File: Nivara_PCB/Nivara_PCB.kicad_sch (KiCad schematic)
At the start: 19 parts, among them J1 NPN_IN, J10 RELAY, J11 FUENTE IN, J12 FUENTE EX, J2 PNP_IN, J3 D_IN, J4 ANALOG_IN, J5 RUN/STOP, J6 NPN_OUT, J7 PNP_OUT, J8 RS485, J9 ANALOG_OUT

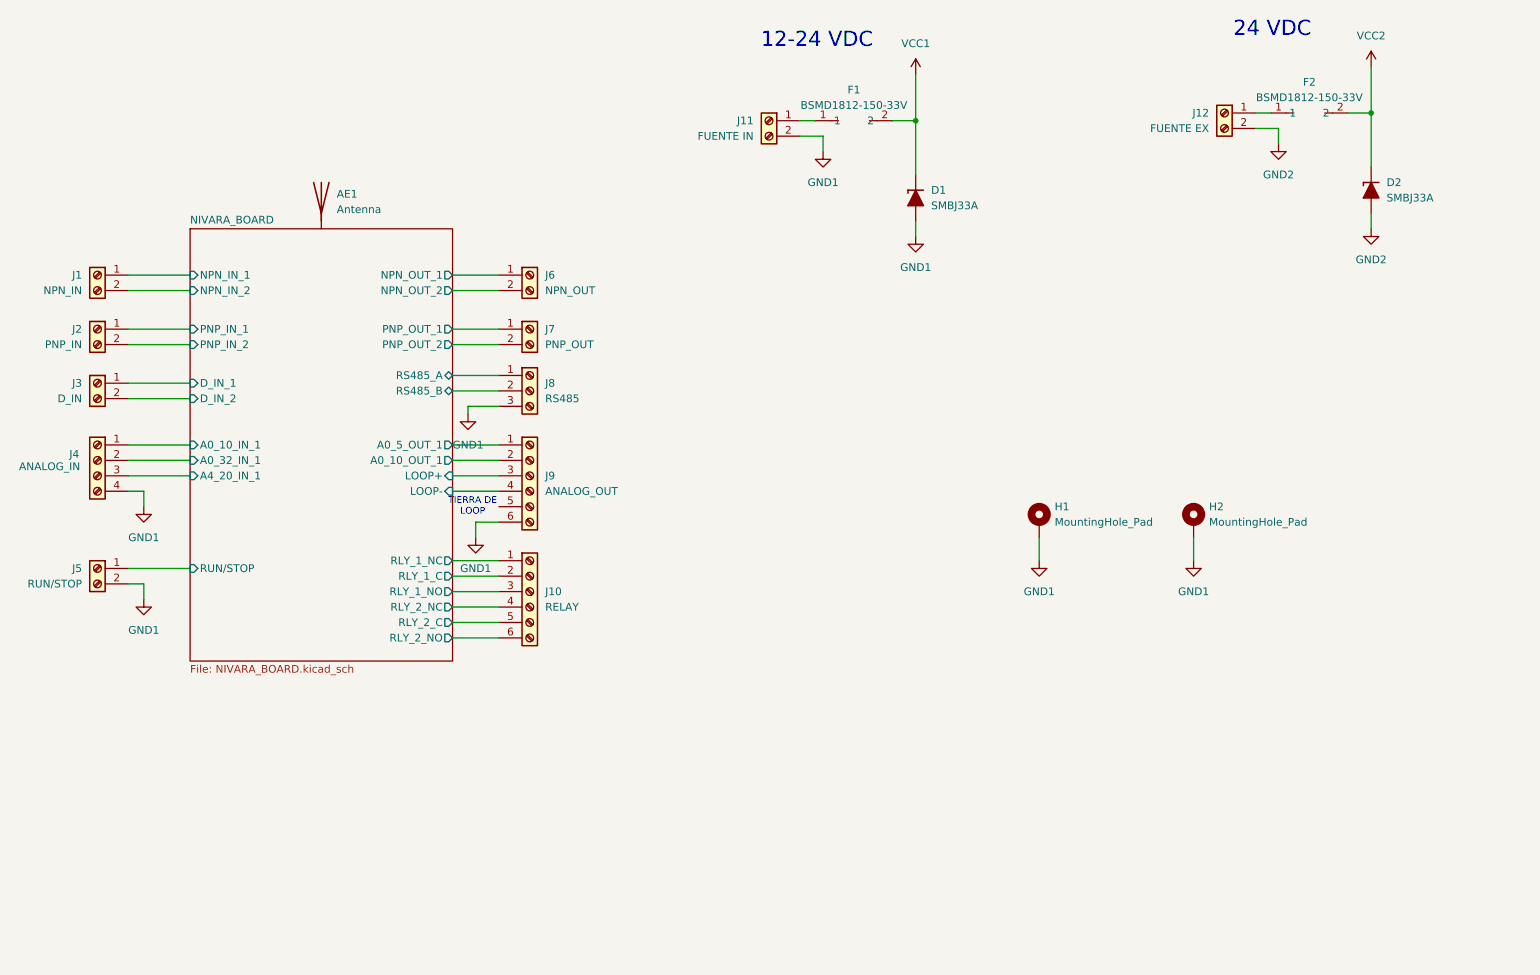
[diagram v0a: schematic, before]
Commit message: New changes to the Nivara PCB schematic files.
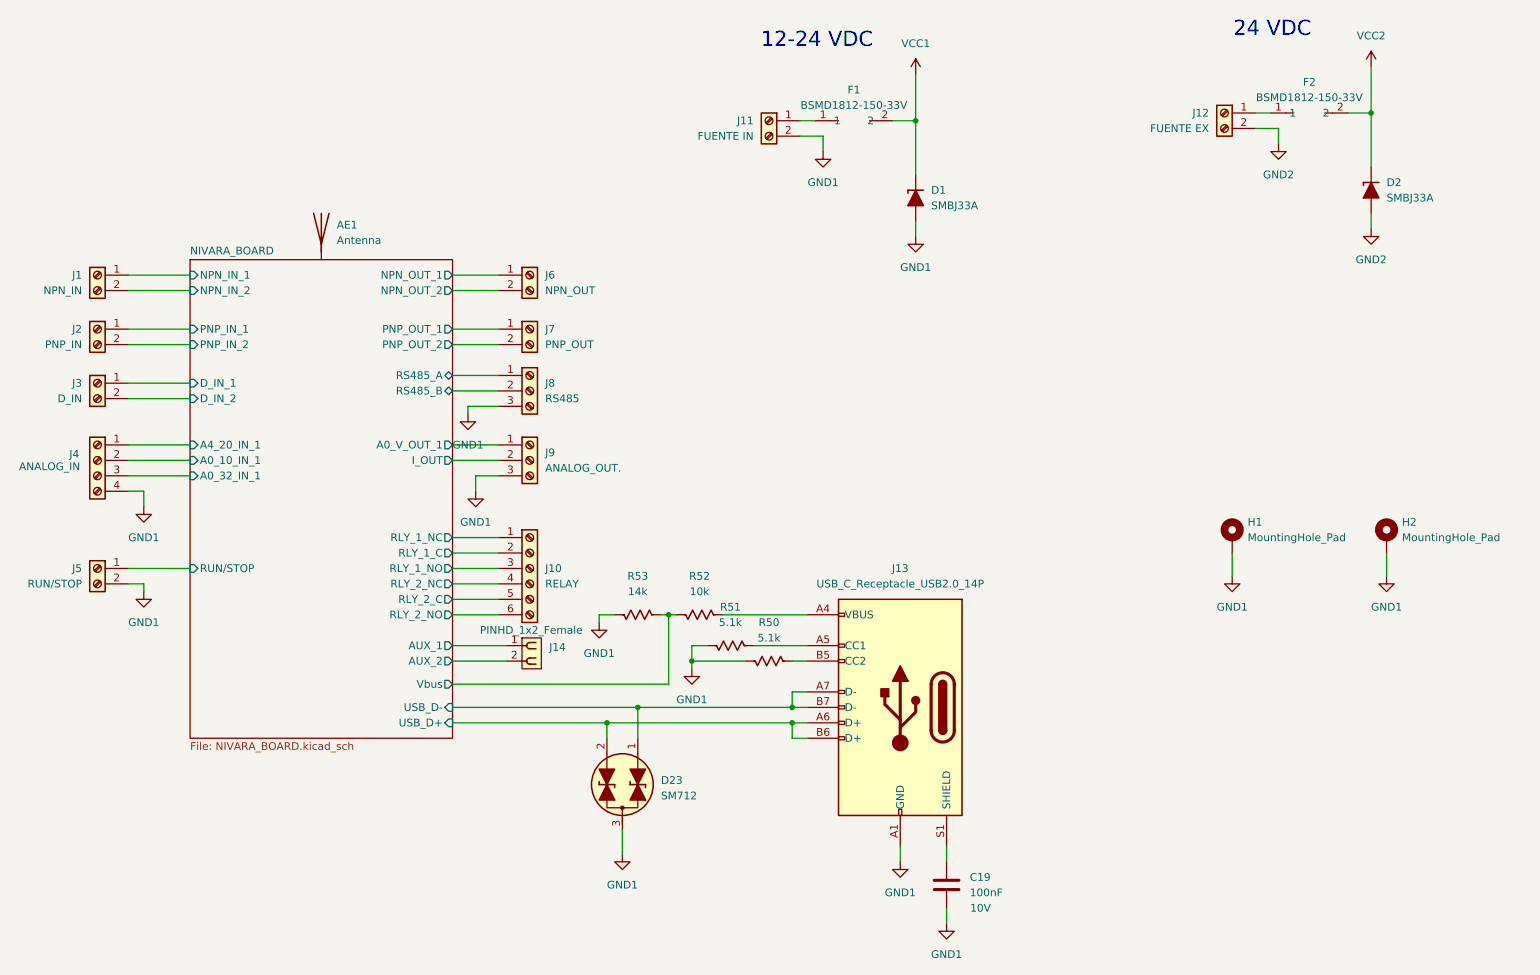
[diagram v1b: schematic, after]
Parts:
- removed J9: ANALOG_OUT, TerminalBlock:TerminalBlock_bornier-6_P5.08mm, symbol Connector:Screw_Terminal_01x06
- added C19: 100nF, PCM_Capacitor_SMD_AKL:C_0603_1608Metric, symbol PCM_Capacitor_US_AKL:C_0603
- added D23: SM712, PCM_Package_TO_SOT_SMD_AKL:SOT-23, symbol PCM_Diode_TVS_AKL:SM712
- added J13: USB_C_Receptacle_USB2.0_14P, symbol Connector:USB_C_Receptacle_USB2.0_14P
- added J14: PINHD_1x2_Female, Connector_PinSocket_2.54mm:PinSocket_1x02_P2.54mm_Vertical, symbol PCM_SL_Pin_Headers:PINHD_1x2_Female
- added J9: ANALOG_OUT., TerminalBlock:TerminalBlock_bornier-3_P5.08mm, symbol Connector:Screw_Terminal_01x03
- added R50, R51: 5.1k, PCM_Resistor_SMD_AKL:R_0805_2012Metric, symbol PCM_Resistor_US_AKL:R_0805
- added R52: 10k, PCM_Resistor_SMD_AKL:R_0603_1608Metric, symbol PCM_Resistor_US_AKL:R_0603
- added R53: 14k, PCM_Resistor_SMD_AKL:R_0603_1608Metric, symbol PCM_Resistor_US_AKL:R_0603
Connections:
- net GND1: now also C19.2, D23.3 (Com), J13.A1 (GND), J13.A12 (GND), J13.B1 (GND), J13.B12 (GND), J9.3 (Pin_3), R50.2, R51.2, R53.1
- net NIVARA_BOARD/A0_10_IN_1: now also J4.2 (Pin_2); no longer J4.1 (Pin_1)
- net NIVARA_BOARD/A0_32_IN_1: now also J4.3 (Pin_3); no longer J4.2 (Pin_2)
- net NIVARA_BOARD/A4_20_IN_1: now also J4.1 (Pin_1); no longer J4.3 (Pin_3)
- new net: J13.A4 (VBUS), J13.A9 (VBUS), J13.B4 (VBUS), J13.B9 (VBUS), R52.2
- new net: J13.A5 (CC1), R51.1
- new net: J13.B5 (CC2), R50.1
- new net: C19.1, J13.S1 (SHIELD)
- new net NIVARA_BOARD/A0_V_OUT_1: J9.1 (Pin_1)
- new net NIVARA_BOARD/AUX_1: J14.1
- new net NIVARA_BOARD/AUX_2: J14.2
- new net NIVARA_BOARD/I_OUT: J9.2 (Pin_2)
- new net NIVARA_BOARD/USB_D+: D23.2 (A2), J13.A6 (D+), J13.B6 (D+)
- new net NIVARA_BOARD/USB_D-: D23.1 (A1), J13.A7 (D-), J13.B7 (D-)
- new net NIVARA_BOARD/Vbus: R52.1, R53.2
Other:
- sheet NIVARA_BOARD ports: added A0_V_OUT_1, AUX_1, AUX_2, I_OUT, USB_D+, USB_D-, Vbus; removed A0_10_OUT_1, A0_5_OUT_1, LOOP+, LOOP-
- note removed: "TIERRA DE LOOP"
- moved on the sheet: AE1, H1, H2, J10
